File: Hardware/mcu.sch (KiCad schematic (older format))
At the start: 40 parts, among them U100 IMXRT1050

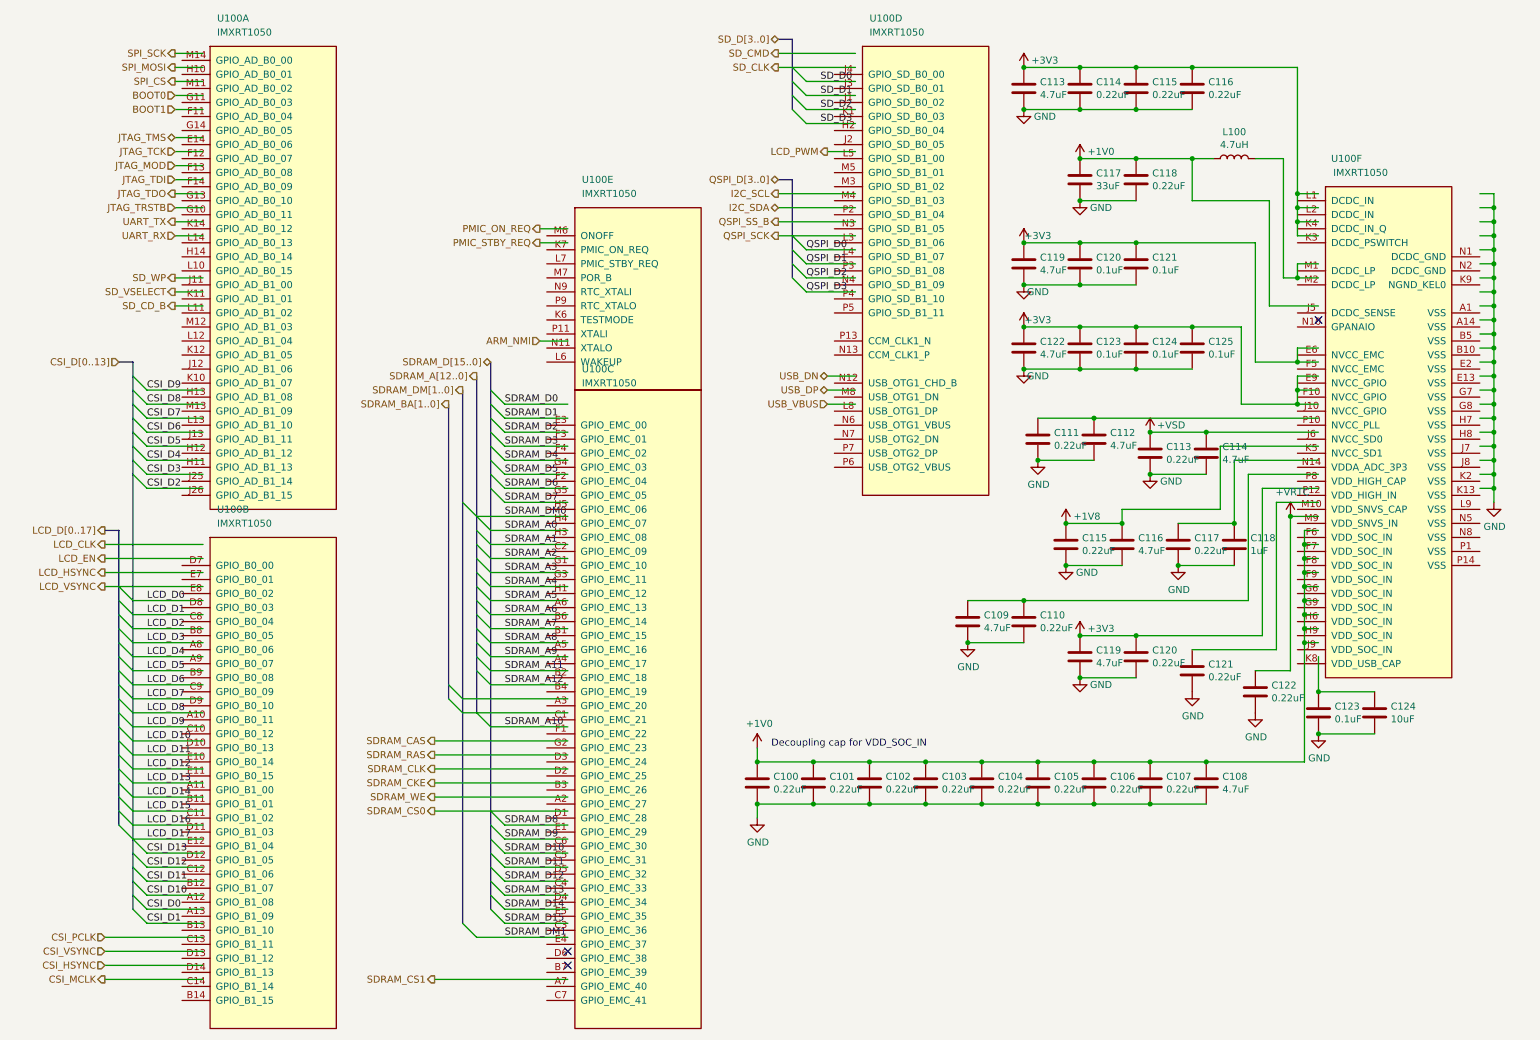
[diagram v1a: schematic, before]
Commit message: pcb: cleanup schematics; working on lcd
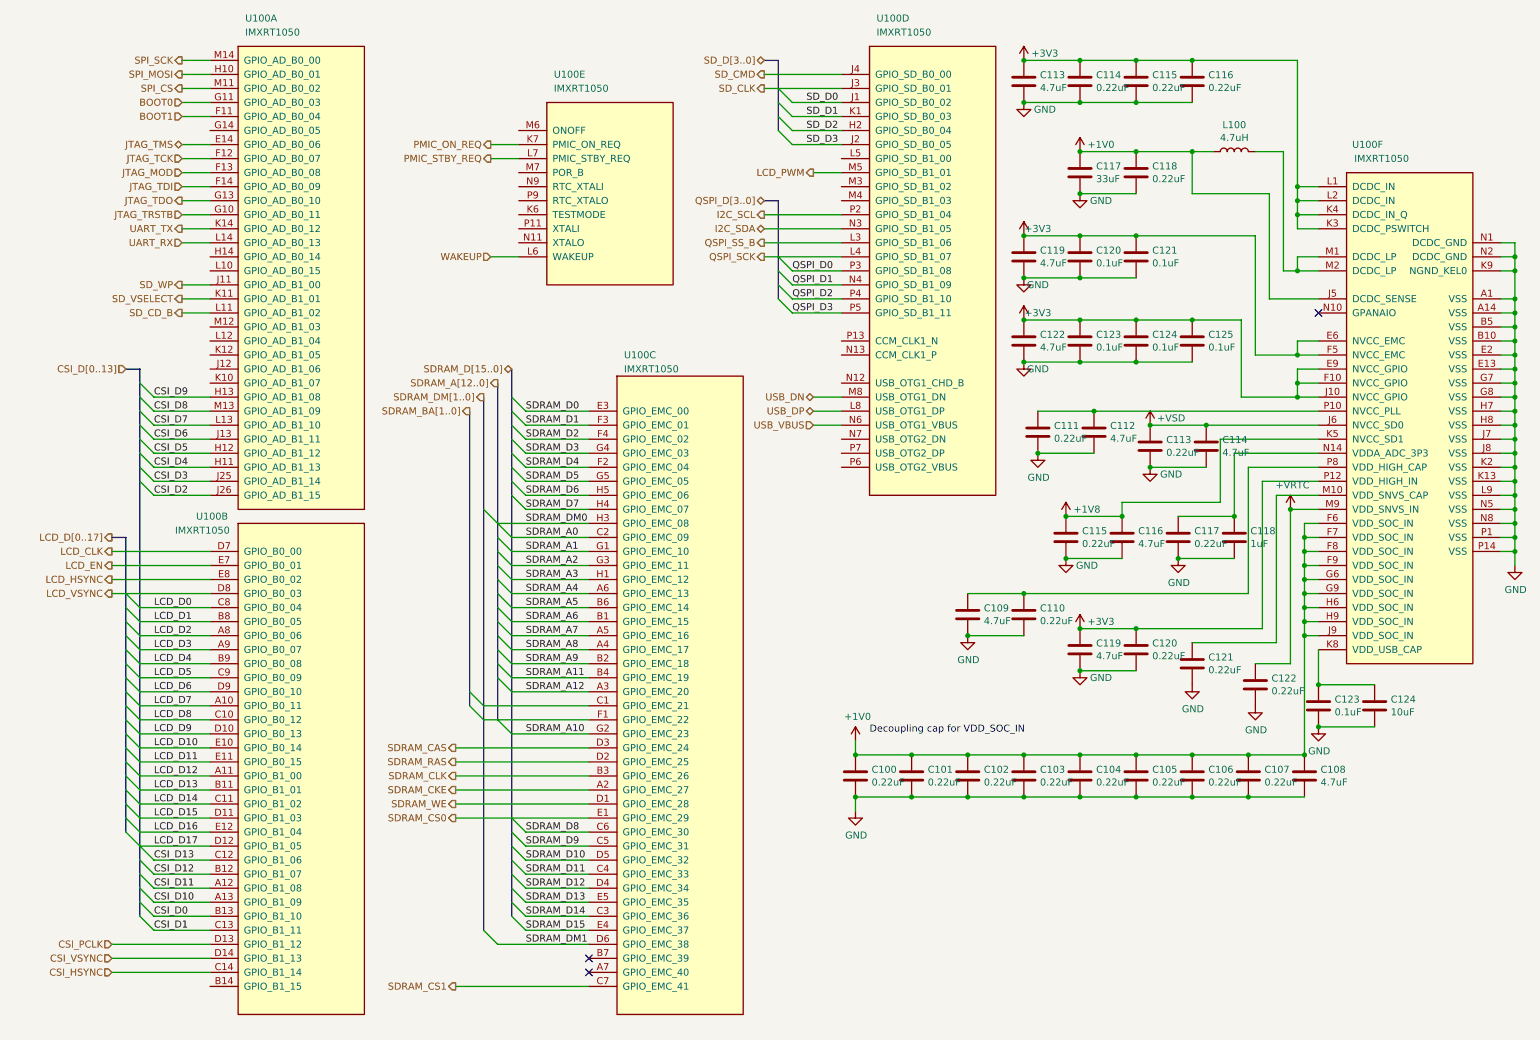
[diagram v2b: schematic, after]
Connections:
- net labels added: WAKEUP
- net labels removed: ARM_NMI, CSI_MCLK
- wire segments 286 -> 284
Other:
- moved on the sheet: C100, C101, C102, C103, C104, C105, C106, C107, C108, C109, C110, C111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

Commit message: pcb: working on power supply
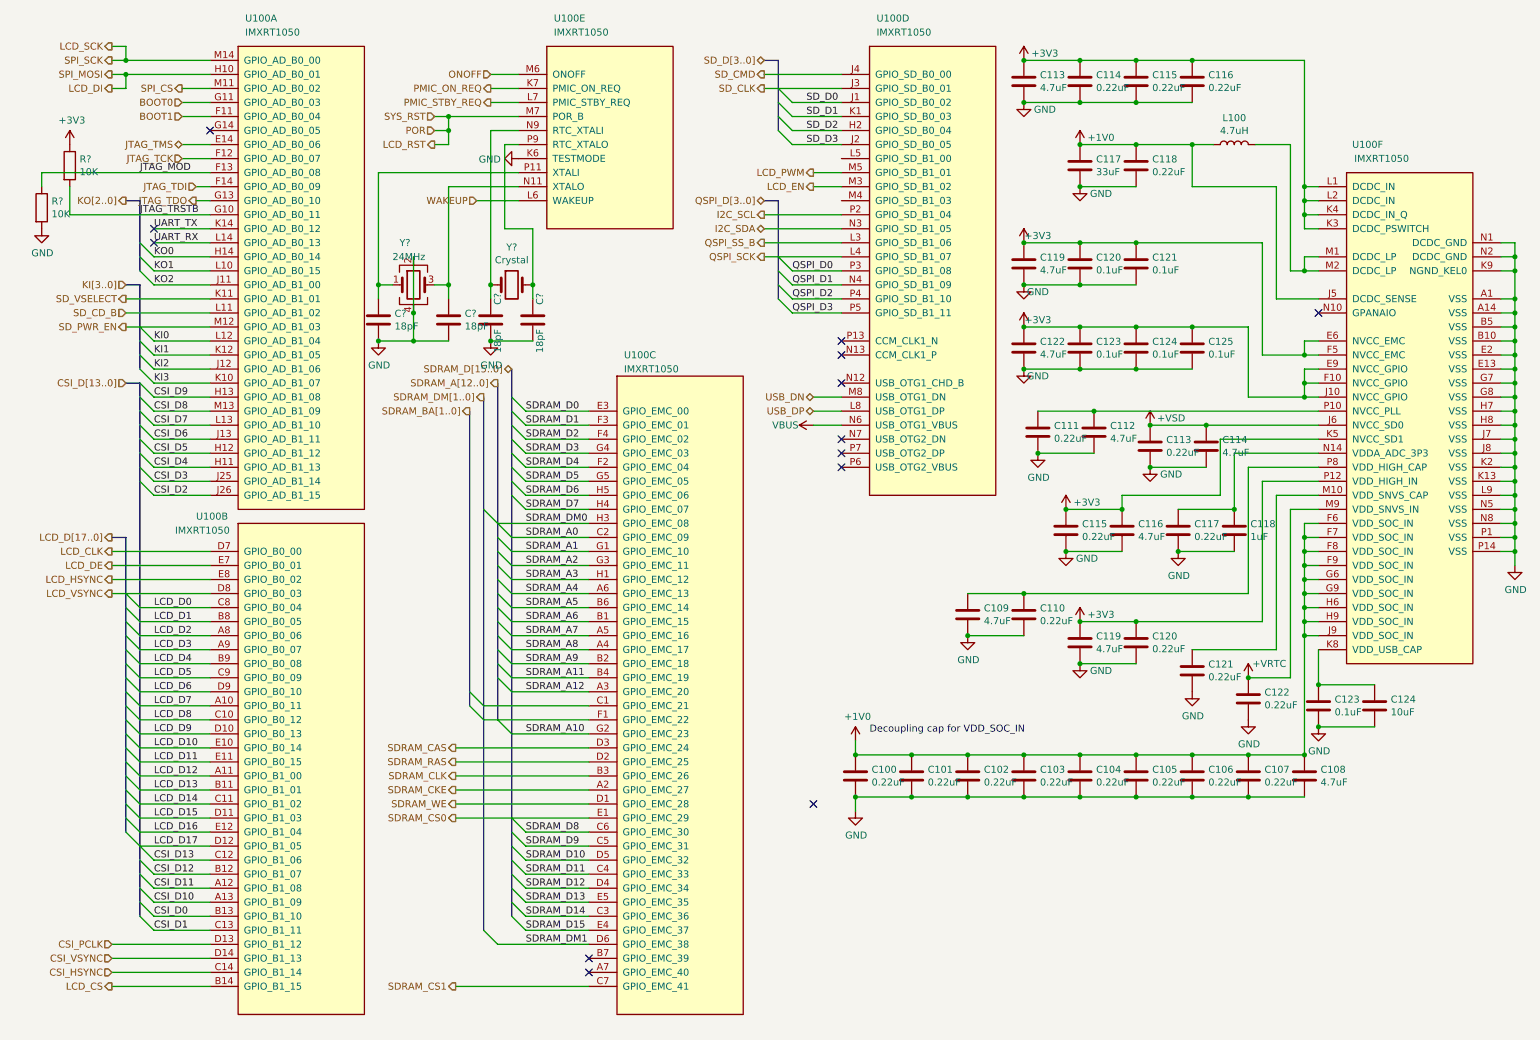
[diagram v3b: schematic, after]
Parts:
- added C? (x4): 18pF, Capacitor_SMD:C_0402_1005Metric, symbol Device:C
- added R? (x2): 10K, symbol Device:R
- added Y?: 24MHz, Oscillator:Oscillator_SMD_Abracon_ASE-4Pin_3.2x2.5mm, symbol Device:Crystal_GND24
- added Y?: Crystal, Crystal:Crystal_SMD_TXC_9HT11-2Pin_2.0x1.2mm_HandSoldering, symbol Device:Crystal
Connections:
- net +1V8 is gone; now on net +3V3: C115.1, C116.1, U100.K5 (NVCC_SD1)
- net +3V3: now also R?.1
- net GND: now also U100.K6 (TESTMODE), C?.1, C?.1, C?.2, C?.2, R?.2, Y?.2, Y?.4
- net JTAG_MOD: now also R?.1
- net JTAG_TRSTB: now also R?.2
- net LCD_EN: now also U100.M3 (GPIO_SD_B1_02); no longer U100.E7 (GPIO_B0_01)
- net LCD_CS: now reaches U100.B14 (GPIO_B1_15)
- net ONOFF: now reaches U100.M6 (ONOFF)
- net LCD_RST: now reaches U100.M7 (POR_B)
- net at U100.N11 (XTALO): now also C?.1, Y?.3
- net at U100.N9 (RTC_XTALI): now also C?.2, Y?.1
- net at U100.P11 (XTALI): now also C?.1, Y?.1
- net at U100.P9 (RTC_XTALO): now also C?.2, Y?.2
- net KO0: now reaches U100.H14 (GPIO_AD_B0_14)
- net KI2: now reaches U100.J12 (GPIO_AD_B1_06)
- net KI3: now reaches U100.K10 (GPIO_AD_B1_07)
- net KI1: now reaches U100.K12 (GPIO_AD_B1_05)
- net KO1: now reaches U100.L10 (GPIO_AD_B0_15)
- net KI0: now reaches U100.L12 (GPIO_AD_B1_04)
- net SD_PWR_EN: now reaches U100.M12 (GPIO_AD_B1_03)
- net SD_WP renamed KO2
- net SPI_MOSI renamed LCD_DI
- net SPI_SCK renamed LCD_SCK
- net USB_VBUS renamed VBUS
- new net LCD_DE: U100.E7 (GPIO_B0_01)
- no-connect marks 3 -> 13
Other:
- moved on the sheet: C115, C116, C117, C118, C119, C120, C121, C122, C123, C124, C125, L100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
